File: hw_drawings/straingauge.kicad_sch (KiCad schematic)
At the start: 167 parts, among them J1 Conn_01x10_Pin, J2 Conn_01x08_Pin, J3 Conn_01x08_Pin, J4 Conn_01x01_Pin, J5 Conn_01x01_Pin, U1 AD7124-8BCPZ, U2 LT8333RDD-PBF, U3 LT3045xMSE, U4 LT3094xDD, U5 LT8333RDD-PBF, U6 Pico, U7 SI8380PM-IU, U8 LT3045xMSE, U9 SIT8008BC-83-33E-2.4576

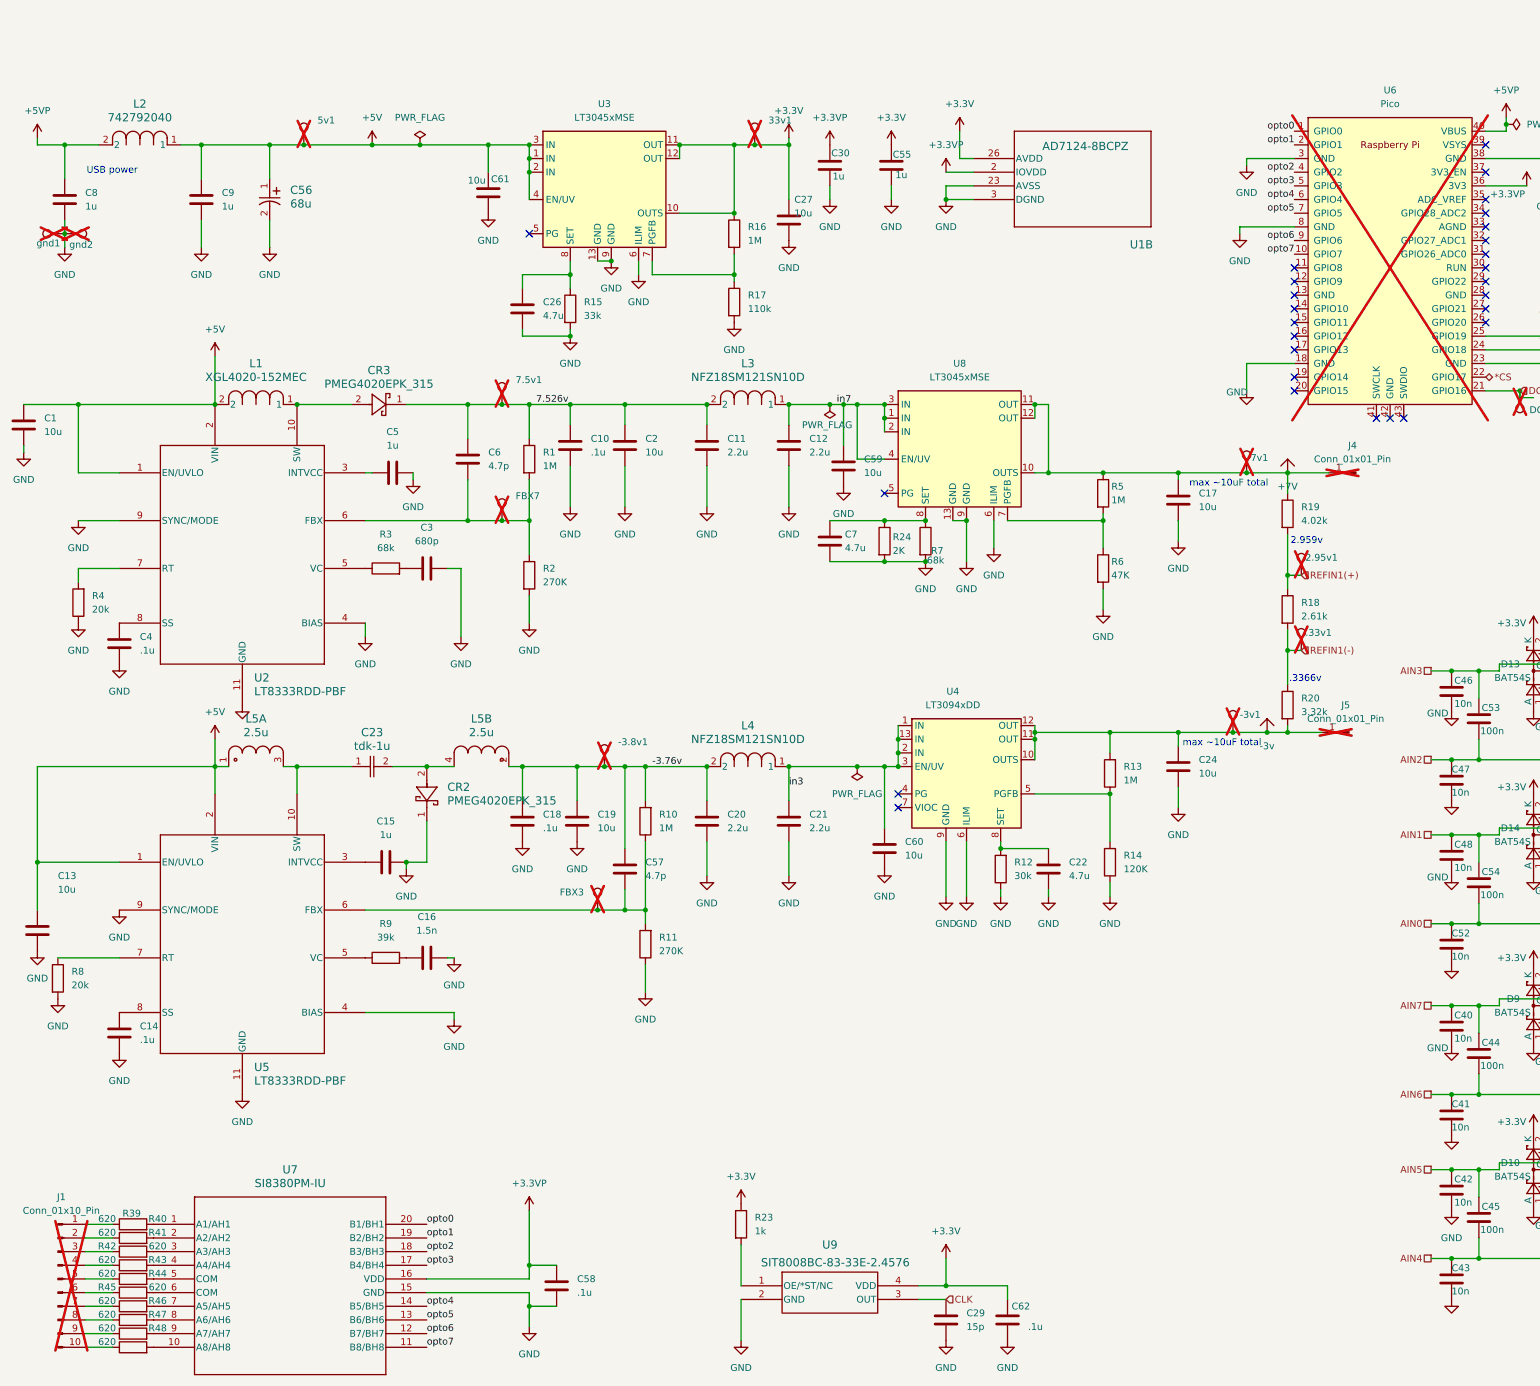
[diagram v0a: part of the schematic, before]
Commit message: full pcb1
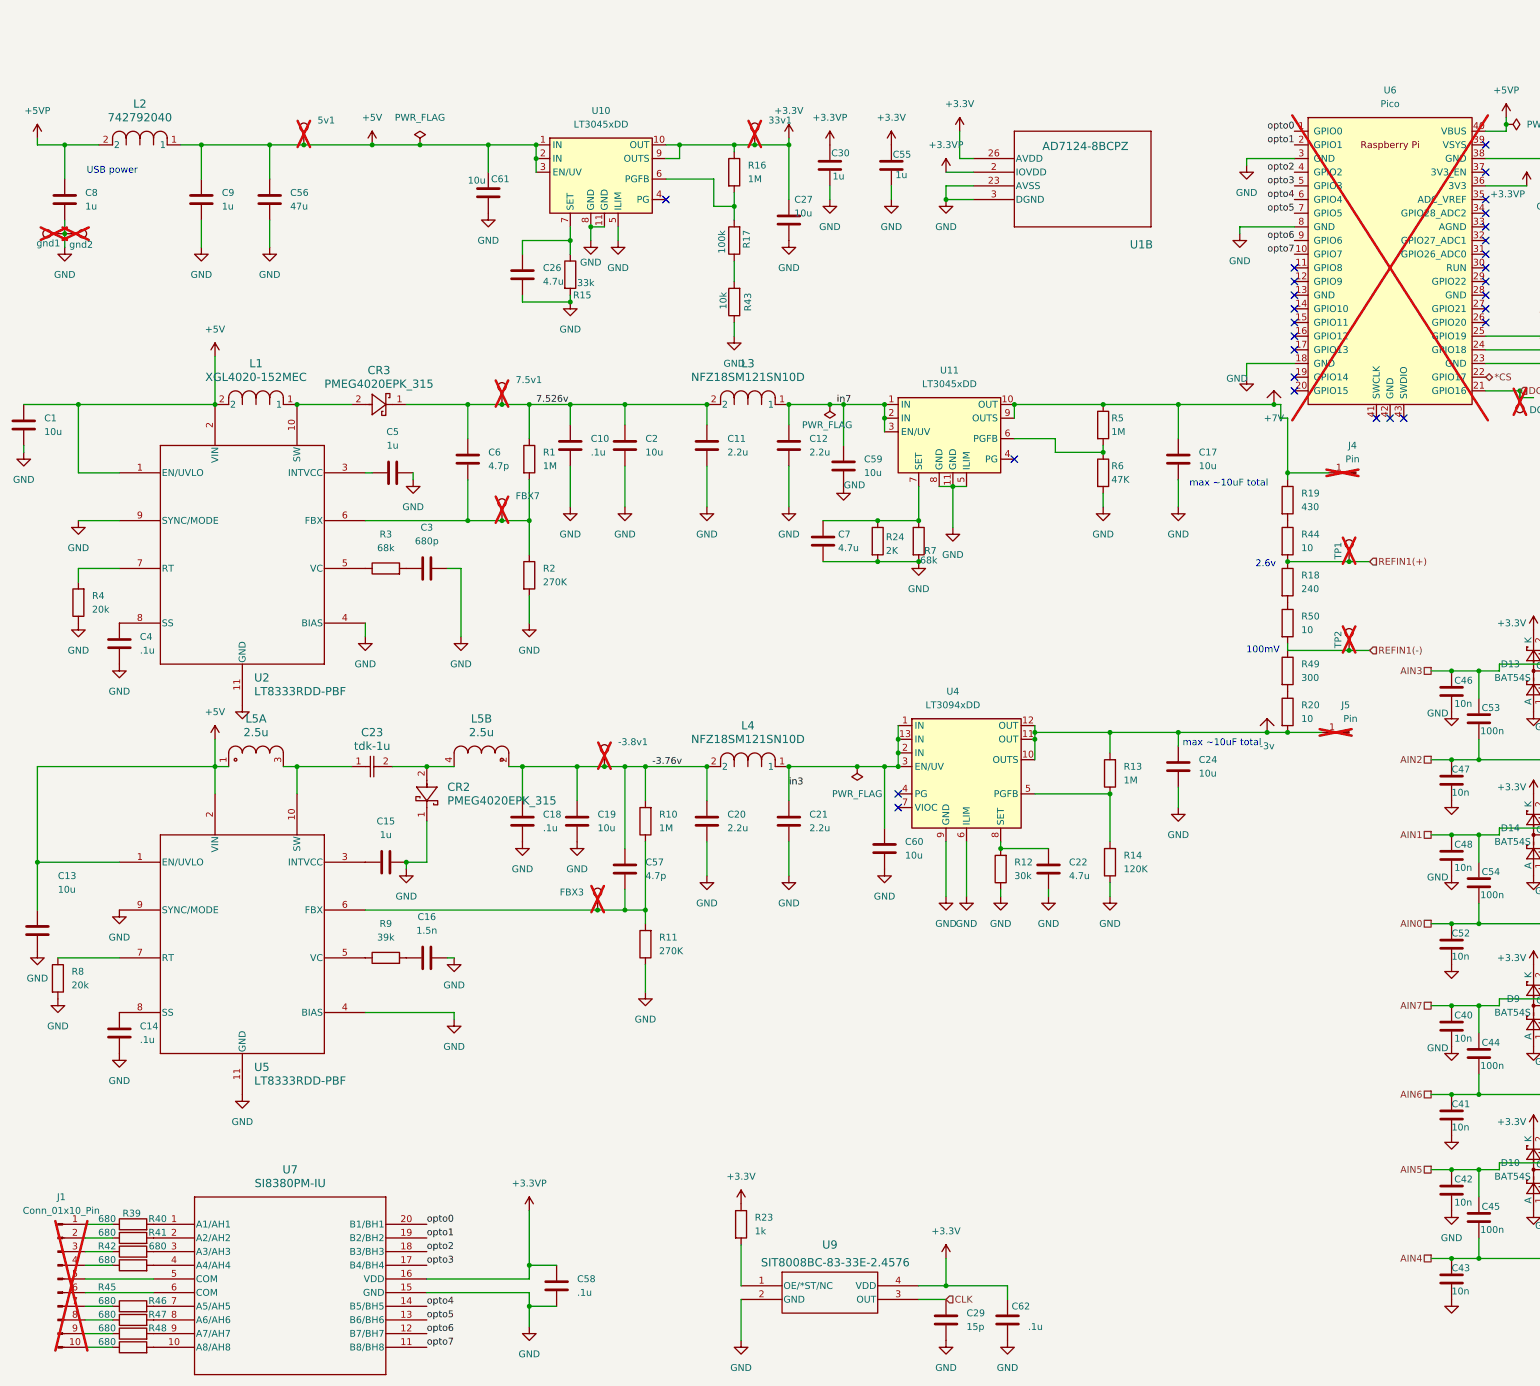
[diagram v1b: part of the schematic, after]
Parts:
- removed -3v1, .33v1, 2.95v1, 7v1: ~, TestPoint:TestPoint_Pad_1.5x1.5mm, symbol Connector:TestPoint
- removed C56: 68u, tant_68u:TAJB_AVX, symbol Tantalum_68u:TAJB686K010RNJ
- removed U3, U8: LT3045xMSE, Package_SO:MSOP-12-1EP_3x4mm_P0.65mm_EP1.65x2.85mm, symbol Regulator3045:LT3045xMSE
- added C56: 47u, Resistor_SMD:R_1206_3216Metric, symbol Device:C
- added R49: 300, Resistor_SMD:R_0805_2012Metric, symbol Device:R
- added R50: 10, Resistor_SMD:R_0805_2012Metric, symbol Device:R
- added TP1, TP2: ~, TestPoint:TestPoint_Pad_1.5x1.5mm, symbol Connector:TestPoint
- added U10, U11: LT3045xDD, Package_DFN_QFN:DFN-10-1EP_3x3mm_P0.5mm_EP1.65x2.38mm, symbol Regulator_Linear_bb:LT3045xDD
- C1, C13, C17, C19, C2, C24, C27, C59, C60, C61: footprint Capacitor_SMD:C_1206_3216Metric -> Capacitor_SMD:C_0805_2012Metric
- C15, C30, C5, C55, C8, C9: footprint Capacitor_SMD:C_0603_1608Metric -> Capacitor_SMD:C_0402_1005Metric
- C29: footprint Capacitor_SMD:C_0201_0603Metric -> Capacitor_SMD:C_0402_1005Metric
- C3: footprint Capacitor_SMD:C_0402_1005Metric -> Capacitor_SMD:C_0603_1608Metric
- J4, J5: value Conn_01x01_Pin -> Pin
- R17: value 110k -> 100k
- R18: value 2.61k -> 240
- R19: value 4.02k -> 430
- R20: value 3.32k -> 10
- R39, R40, R41, R42, R45, R46, R47, R48: value 620 -> 680
- R43: value 620 -> 10k
- R44: value 620 -> 10
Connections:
- net +3.3V: now also U10.10 (OUT), U10.9 (OUTS)
- net +5V: now also C56.1, U10.1 (IN), U10.2 (IN), U10.3 (EN/UV)
- net +7V: now also U11.10 (OUT), U11.9 (OUTS)
- net GND: now also R43.1, C56.2, U10.11 (GND), U10.5 (ILIM), U10.8 (GND), U11.11 (GND), U11.5 (ILIM), U11.8 (GND); no longer R17.2
- net REFIN1(+): now also R44.2, TP1.1; no longer R19.2
- net REFIN1(-): now also R49.1, R50.2, TP2.1; no longer R18.2, R20.1
- net in7: now also U11.1 (IN), U11.2 (IN), U11.3 (EN/UV)
- net at R5.2, R6.1: now also U11.6 (PGFB)
- net at C7.1, R24.1, R7.1: now also U11.7 (SET)
- net at U7.5 (COM): now also J1.5 (Pin_5); no longer R43.2
- net at U7.6 (COM): now also J1.6 (Pin_6); no longer R44.2
- net at R44.1: now also R19.2; no longer J1.6 (Pin_6)
- net at C26.1, R15.1: now also U10.7 (SET)
- net at R17.1: now also R43.2; no longer R16.2
- new net: R20.1, R49.2
- new net: R18.2, R50.1
- new net: R16.2, R17.2, U10.6 (PGFB)
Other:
- note added: "100mV"
- note added: "2.6v"
- note removed: ".3366v"
- note removed: "2.959v"
- moved on the sheet: C17, C26, C7, R15, R16, R17, R18, R19, R20, R24, R5, R6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
